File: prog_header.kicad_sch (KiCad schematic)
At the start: 2 parts

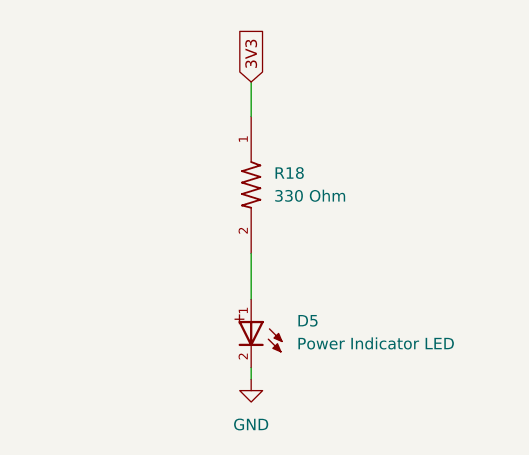
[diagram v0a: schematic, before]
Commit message: PCB tentative finished
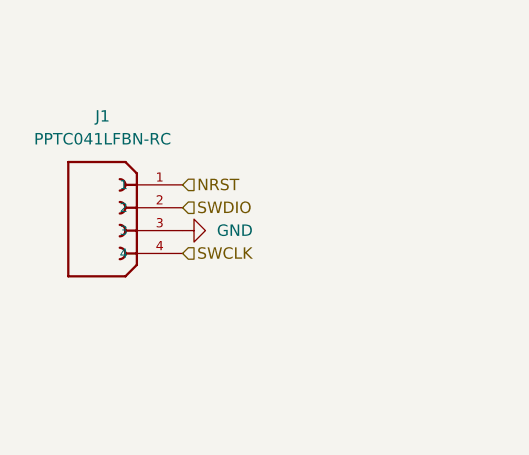
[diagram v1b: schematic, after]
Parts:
- removed D5: Power Indicator LED, LED_WL-TMRC_5MM:WL-TMRC_5MM, symbol PowerIndicatorLED_WL-TMRC_5MM:WL-TMRC_5MM
- removed R18: 330 Ohm, 330_ohm_RC0603FR-07330RL:RESC1607X60N, symbol 330_ohm_RC0603FR-07330RL:RC0603FR-07330RL
- added J1: PPTC041LFBN-RC, Connector_01x04_PPTC041LFBN-RC:SULLINS_PPTC041LFBN-RC, symbol Connector_01x04_PPTC041LFBN-RC:PPTC041LFBN-RC
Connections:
- net GND: now also J1.3
- new net NRST: J1.1
- new net SWCLK: J1.4
- new net SWDIO: J1.2
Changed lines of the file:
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@@
 	(generator_version "9.0")
 	(paper "A4")
-	(wire
-		(pts
-			(xy 132.08 107.95) (xy 132.08 109.22)
-		)
-		(stroke
-			(width 0)
-			(type default)
-		)
-	)
-	(wire
-		(pts
-			(xy 132.08 95.25) (xy 132.08 100.33)
-		)
-		(stroke
-			(width 0)
-			(type default)
-		)
-	)
-	(wire
-		(pts
-			(xy 132.08 76.2) (xy 132.08 80.01)
-		)
-		(stroke
-			(width 0)
-			(type default)
-		)
-	)
-	(global_label "3V3"
+	(hierarchical_label "SWDIO"
 		(shape input)
-		(at 132.08 76.2 90)
-		(fields_autoplaced yes)
+		(at 124.46 90.17 0)
 		(effects
 			(font
@@
 			(justify left)
 		)
-		(property "Intersheetrefs" "${INTERSHEET_REFS}"
-			(at 132.08 69.7072 90)
-			(effects
-				(font
-					(size 1.27 1.27)
-				)
-				(justify left)
-				(hide yes)
-			)
+	)
+	(hierarchical_label "NRST"
+		(shape input)
+		(at 124.46 87.63 0)
+		(effects
+			(font
+				(size 1.27 1.27)
+			)
+			(justify left)
+		)
+	)
+	(hierarchical_label "SWCLK"
+		(shape input)
+		(at 124.46 95.25 0)
+		(effects
+			(font
+				(size 1.27 1.27)
+			)
+			(justify left)
 		)
 	)
 	(symbol
 		(lib_id "power:GND")
-		(at 132.08 109.22 0)
+		(at 124.46 92.71 90)
 		(unit 1)
 		(exclude_from_sim no)
@@
 		(dnp no)
 		(fields_autoplaced yes)
-		(property "Reference" "#PWR018"
-			(at 132.08 115.57 0)
+		(property "Reference" "#PWR04"
+			(at 130.81 92.71 0)
 			(effects
 				(font
@@
 		)
 		(property "Value" "GND"
-			(at 132.08 114.3 0)
-			(effects
-				(font
-					(size 1.27 1.27)
-				)
+			(at 128.27 92.7099 90)
+			(effects
+				(font
+					(size 1.27 1.27)
+				)
+				(justify right)
 			)
 		)
 		(property "Footprint" ""
-			(at 132.08 109.22 0)
+			(at 124.46 92.71 0)
 			(effects
 				(font
@@
 		)
 		(property "Datasheet" ""
-			(at 132.08 109.22 0)
+			(at 124.46 92.71 0)
 			(effects
 				(font
@@
 		)
 		(property "Description" "Power symbol creates a global label with name \"GND\" , ground"
-			(at 132.08 109.22 0)
+			(at 124.46 92.71 0)
 			(effects
 				(font
@@
 		(instances
 			(project "IREmitter"
-				(path "/d311851a-8b0b-4acf-b2e7-1b968b2adbe7/7e232de8-a719-408b-a25a-fa0b7a2171cb"
-					(reference "#PWR018")
+				(path "/d311851a-8b0b-4acf-b2e7-1b968b2adbe7/bb69d768-066e-4777-a725-fdf4f103ecbb"
+					(reference "#PWR04")
 					(unit 1)
 				)
@@
 	)
 	(symbol
-		(lib_id "PowerIndicatorLED_WL-TMRC_5MM:WL-TMRC_5MM")
-		(at 132.08 105.41 270)
+		(lib_id "Connector_01x04_PPTC041LFBN-RC:PPTC041LFBN-RC")
+		(at 119.38 90.17 0)
 		(unit 1)
 		(exclude_from_sim no)
@@
 		(dnp no)
 		(fields_autoplaced yes)
-		(property "Reference" "D5"
-			(at 137.16 102.769 90)
-			(effects
-				(font
-					(size 1.27 1.27)
-				)
-				(justify left)
-			)
-		)
-		(property "Value" "Power Indicator LED"
-			(at 137.16 105.309 90)
-			(effects
-				(font
-					(size 1.27 1.27)
-				)
-				(justify left)
-			)
-		)
-		(property "Footprint" "LED_WL-TMRC_5MM:WL-TMRC_5MM"
-			(at 132.08 105.41 0)
+		(property "Reference" "J1"
+			(at 115.57 80.01 0)
+			(effects
+				(font
+					(size 1.27 1.27)
+				)
+			)
+		)
+		(property "Value" "PPTC041LFBN-RC"
+			(at 115.57 82.55 0)
+			(effects
+				(font
+					(size 1.27 1.27)
+				)
+			)
+		)
+		(property "Footprint" "Connector_01x04_PPTC041LFBN-RC:SULLINS_PPTC041LFBN-RC"
+			(at 119.38 90.17 0)
 			(effects
 				(font
@@
 		)
 		(property "Datasheet" ""
-			(at 132.08 105.41 0)
+			(at 119.38 90.17 0)
 			(effects
 				(font
@@
 		)
 		(property "Description" ""
-			(at 132.08 105.41 0)
-			(effects
-				(font
-					(size 1.27 1.27)
-				)
-				(hide yes)
-			)
+			(at 119.38 90.17 0)
+			(effects
+				(font
+					(size 1.27 1.27)
+				)
+				(hide yes)
+			)
+		)
+		(property "DigiKey_Part_Number" "S7002-ND"
+			(at 119.38 90.17 0)
+			(effects
+				(font
+					(size 1.27 1.27)
+				)
+				(justify bottom)
+				(hide yes)
+			)
+		)
+		(property "SnapEDA_Link" "https://www.snapeda.com/parts/PPTC041LFBN-RC/Sullins/view-part/?ref=snap"
+			(at 119.38 90.17 0)
+			(effects
+				(font
+					(size 1.27 1.27)
+				)
+				(justify bottom)
+				(hide yes)
+			)
+		)
+		(property "MAXIMUM_PACKAGE_HEIGHT" "8.5mm"
+			(at 119.38 90.17 0)
+			(effects
+				(font
+					(size 1.27 1.27)
+				)
+				(justify bottom)
+				(hide yes)
+			)
+		)
+		(property "Package" "None"
+			(at 119.38 90.17 0)
+			(effects
+				(font
+					(size 1.27 1.27)
+				)
+				(justify bottom)
+				(hide yes)
+			)
+		)
+		(property "Check_prices" "https://www.snapeda.com/parts/PPTC041LFBN-RC/Sullins/view-part/?ref=eda"
+			(at 119.38 90.17 0)
+			(effects
+				(font
+					(size 1.27 1.27)
+				)
+				(justify bottom)
+				(hide yes)
+			)
+		)
+		(property "STANDARD" "Manufacturer Recommendations"
+			(at 119.38 90.17 0)
+			(effects
+				(font
+					(size 1.27 1.27)
+				)
+				(justify bottom)
+				(hide yes)
+			)
+		)
+		(property "PARTREV" "J - 04/15/2015"
+			(at 119.38 90.17 0)
+			(effects
+				(font
+					(size 1.27 1.27)
+				)
+				(justify bottom)
+				(hide yes)
+			)
+		)
+		(property "MF" "Sullins Connector"
+			(at 119.38 90.17 0)
+			(effects
+				(font
+					(size 1.27 1.27)
+				)
+				(justify bottom)
+				(hide yes)
+			)
+		)
+		(property "MP" "PPTC041LFBN-RC"
+			(at 119.38 90.17 0)
+			(effects
+				(font
+					(size 1.27 1.27)
+				)
+				(justify bottom)
+				(hide yes)
+			)
+		)
+		(property "Description_1" "4 Position Header Connector 0.100 (2.54mm) Through Hole Tin"
+			(at 119.38 90.17 0)
+			(effects
+				(font
+					(size 1.27 1.27)
+				)
+				(justify bottom)
+				(hide yes)
+			)
+		)
+		(property "MANUFACTURER" "SULLINS"
+			(at 119.38 90.17 0)
+			(effects
+				(font
+					(size 1.27 1.27)
+				)
+				(justify bottom)
+				(hide yes)
+			)
+		)
+		(pin "2"
+		)
+		(pin "3"
+		)
+		(pin "4"
 		)
 		(pin "1"
-		)
-		(pin "2"
 		)
 		(instances
 			(project "IREmitter"
-				(path "/d311851a-8b0b-4acf-b2e7-1b968b2adbe7/7e232de8-a719-408b-a25a-fa0b7a2171cb"
-					(reference "D5")
+				(path "/d311851a-8b0b-4acf-b2e7-1b968b2adbe7/bb69d768-066e-4777-a725-fdf4f103ecbb"
+					(reference "J1")
 					(unit 1)
 				)
-			)
-		)
-	)
-	(symbol
-		(lib_id "330_ohm_RC0603FR-07330RL:RC0603FR-07330RL")
-		(at 132.08 87.63 270)
-		(unit 1)
-		(exclude_from_sim no)
-		(in_bom yes)
-		(on_board yes)
-		(dnp no)
-		(fields_autoplaced yes)
-		(property "Reference" "R18"
-			(at 134.62 86.3599 90)
-			(effects
-				(font
-					(size 1.27 1.27)
-				)
-				(justify left)
-			)
-		)
-		(property "Value" "330 Ohm"
-			(at 134.62 88.8999 90)
-			(effects
-				(font
-					(size 1.27 1.27)
-				)
-				(justify left)
-			)
-		)
-		(property "Footprint" "330_ohm_RC0603FR-07330RL:RESC1607X60N"
-			(at 132.08 87.63 0)
-			(effects
-				(font
-					(size 1.27 1.27)
-				)
-				(justify bottom)
-				(hide yes)
-			)
-		)
-		(property "Datasheet" ""
-			(at 132.08 87.63 0)
-			(effects
-				(font
-					(size 1.27 1.27)
-				)
-				(hide yes)
-			)
-		)
-		(property "Description" ""
-			(at 132.08 87.63 0)
-			(effects
-				(font
-					(size 1.27 1.27)
-				)
-				(hide yes)
-			)
-		)
-		(property "DigiKey_Part_Number" "311-330HRCT-ND"
-			(at 132.08 87.63 0)
-			(effects
-				(font
-					(size 1.27 1.27)
-				)
-				(justify bottom)
-				(hide yes)
-			)
-		)
-		(property "SnapEDA_Link" "https://www.snapeda.com/parts/RC0603FR-07330RL/Yageo/view-part/?ref=snap"
-			(at 132.08 87.63 0)
-			(effects
-				(font
-					(size 1.27 1.27)
-				)
-				(justify bottom)
-				(hide yes)
-			)
-		)
-		(property "Description_1" "330 Ohms ±1% 0.1W, 1/10W Chip Resistor 0603 (1608 Metric) Moisture Resistant Thick Film"
-			(at 132.08 87.63 0)
-			(effects
-				(font
-					(size 1.27 1.27)
-				)
-				(justify bottom)
-				(hide yes)
-			)
-		)
-		(property "MF" "Yageo"
-			(at 132.08 87.63 0)
-			(effects
-				(font
-					(size 1.27 1.27)
-				)
-				(justify bottom)
-				(hide yes)
-			)
-		)
-		(property "Package" "0603 Yageo"
-			(at 132.08 87.63 0)
-			(effects
-				(font
-					(size 1.27 1.27)
-				)
-				(justify bottom)
-				(hide yes)
-			)
-		)
-		(property "Check_prices" "https://www.snapeda.com/parts/RC0603FR-07330RL/Yageo/view-part/?ref=eda"
-			(at 132.08 87.63 0)
-			(effects
-				(font
-					(size 1.27 1.27)
-				)
-				(justify bottom)
-				(hide yes)
-			)
-		)
-		(property "MP" "RC0603FR-07330RL"
-			(at 132.08 87.63 0)
-			(effects
-				(font
-					(size 1.27 1.27)
-				)
-				(justify bottom)
-				(hide yes)
-			)
-		)
-		(pin "2"
-		)
-		(pin "1"
-		)
-		(instances
-			(project "IREmitter"
-				(path "/d311851a-8b0b-4acf-b2e7-1b968b2adbe7/7e232de8-a719-408b-a25a-fa0b7a2171cb"
-					(reference "R18")
-					(unit 1)
-				)
